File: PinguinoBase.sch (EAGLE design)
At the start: 27 parts, among them IC1 7805, Q1 20MHz, X1 

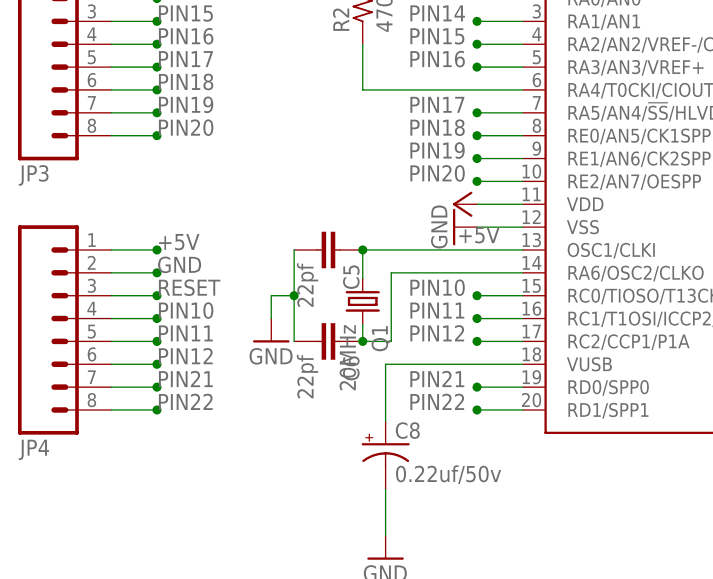
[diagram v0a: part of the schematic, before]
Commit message: Update 3v4
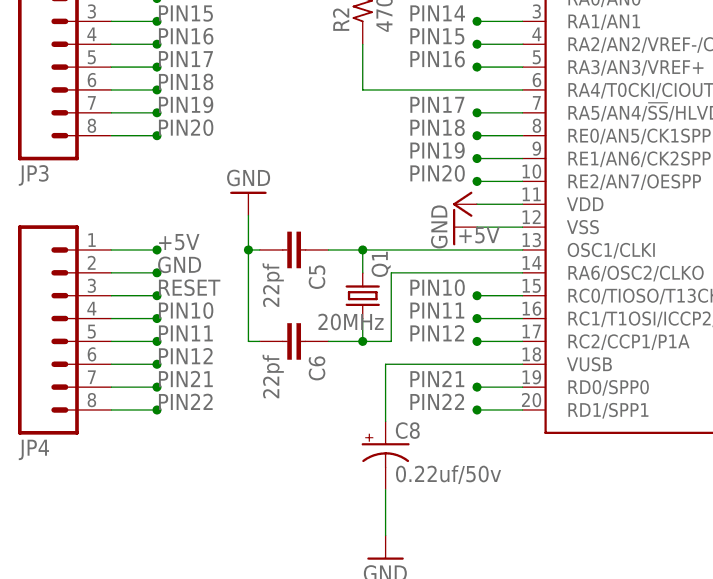
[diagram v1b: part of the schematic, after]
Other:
- moved on the sheet: C5, C6, Q1
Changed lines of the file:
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@@
 <setting verticaltext="up"/>
 </settings>
-<grid distance="0.05" unitdist="inch" unit="inch" style="lines" multiple="1" display="no" altdistance="0.01" altunitdist="inch" altunit="inch"/>
+<grid distance="0.05" unitdist="inch" unit="inch" style="lines" multiple="1" display="yes" altdistance="0.01" altunitdist="inch" altunit="inch"/>
 <layers>
 <layer number="1" name="Top" color="4" fill="1" visible="no" active="no"/>
@@
 <instance part="P+5" gate="1" x="-58.42" y="88.9"/>
 <instance part="GND9" gate="1" x="-58.42" y="71.12"/>
-<instance part="Q1" gate="G$1" x="-48.26" y="19.685" rot="R270"/>
-<instance part="C5" gate="G$1" x="-53.34" y="25.4" rot="R270"/>
-<instance part="C6" gate="G$1" x="-53.34" y="15.24" rot="R270"/>
+<instance part="Q1" gate="G$1" x="-48.26" y="20.32" smashed="yes" rot="R270">
+<attribute name="NAME" x="-47.244" y="25.4" size="1.778" layer="95" rot="R270"/>
+<attribute name="VALUE" x="-53.34" y="16.51" size="1.778" layer="96"/>
+</instance>
+<instance part="C5" gate="G$1" x="-57.15" y="25.4" rot="R270"/>
+<instance part="C6" gate="G$1" x="-57.15" y="15.24" rot="R270"/>
 <instance part="GND11" gate="1" x="-45.72" y="-8.89"/>
 <instance part="RESET" gate="1" x="30.48" y="71.12" smashed="yes" rot="MR270">
@@
 <instance part="P+1" gate="1" x="-71.12" y="88.9"/>
 <instance part="GND1" gate="1" x="-71.12" y="71.12"/>
-<instance part="GND10" gate="1" x="-58.42" y="15.24"/>
+<instance part="GND10" gate="1" x="-60.96" y="31.75" rot="R180"/>
 <instance part="X1" gate="-1" x="-60.96" y="129.54"/>
 <instance part="X1" gate="-2" x="-60.96" y="124.46"/>
@@
 </segment>
 <segment>
-<wire x1="-58.42" y1="17.78" x2="-58.42" y2="20.32" width="0.1524" layer="91"/>
-<wire x1="-55.88" y1="25.4" x2="-55.88" y2="20.32" width="0.1524" layer="91"/>
-<wire x1="-55.88" y1="20.32" x2="-55.88" y2="15.24" width="0.1524" layer="91"/>
-<wire x1="-58.42" y1="20.32" x2="-55.88" y2="20.32" width="0.1524" layer="91"/>
-<junction x="-55.88" y="20.32"/>
+<wire x1="-60.96" y1="29.21" x2="-60.96" y2="25.4" width="0.1524" layer="91"/>
+<wire x1="-59.69" y1="25.4" x2="-60.96" y2="25.4" width="0.1524" layer="91"/>
+<wire x1="-60.96" y1="25.4" x2="-60.96" y2="15.24" width="0.1524" layer="91"/>
+<wire x1="-60.96" y1="15.24" x2="-59.69" y2="15.24" width="0.1524" layer="91"/>
+<junction x="-60.96" y="25.4"/>
 <pinref part="GND10" gate="1" pin="GND"/>
 <pinref part="C5" gate="G$1" pin="2"/>
@@
 <segment>
 <wire x1="-30.48" y1="25.4" x2="-48.26" y2="25.4" width="0.1524" layer="91"/>
-<wire x1="-48.26" y1="25.4" x2="-48.26" y2="22.225" width="0.1524" layer="91"/>
+<pinref part="18F4550" gate="G$1" pin="OSC1/CLKI"/>
+<pinref part="C5" gate="G$1" pin="1"/>
+<pinref part="Q1" gate="G$1" pin="1"/>
+<wire x1="-48.26" y1="25.4" x2="-52.07" y2="25.4" width="0.1524" layer="91"/>
+<wire x1="-48.26" y1="22.86" x2="-48.26" y2="25.4" width="0.1524" layer="91"/>
 <junction x="-48.26" y="25.4"/>
-<pinref part="18F4550" gate="G$1" pin="OSC1/CLKI"/>
-<pinref part="Q1" gate="G$1" pin="1"/>
-<pinref part="C5" gate="G$1" pin="1"/>
 </segment>
 </net>
 <net name="N$5" class="0">
 <segment>
-<wire x1="-48.26" y1="17.145" x2="-48.26" y2="15.24" width="0.1524" layer="91"/>
+<wire x1="-52.07" y1="15.24" x2="-48.26" y2="15.24" width="0.1524" layer="91"/>
 <wire x1="-48.26" y1="15.24" x2="-45.085" y2="15.24" width="0.1524" layer="91"/>
 <wire x1="-45.085" y1="15.24" x2="-45.085" y2="22.86" width="0.1524" layer="91"/>
 <wire x1="-45.085" y1="22.86" x2="-30.48" y2="22.86" width="0.1524" layer="91"/>
-<junction x="-48.26" y="15.24"/>
-<pinref part="Q1" gate="G$1" pin="2"/>
 <pinref part="18F4550" gate="G$1" pin="RA6/OSC2/CLKO"/>
 <pinref part="C6" gate="G$1" pin="1"/>
+<pinref part="Q1" gate="G$1" pin="2"/>
+<wire x1="-48.26" y1="17.78" x2="-48.26" y2="15.24" width="0.1524" layer="91"/>
+<junction x="-48.26" y="15.24"/>
 </segment>
 </net>
